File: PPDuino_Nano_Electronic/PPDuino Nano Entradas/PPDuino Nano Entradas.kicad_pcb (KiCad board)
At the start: 2 copper layers, 51.6 x 59.4 mm, 27 parts, among them J10 PWR_OUT, J11 INPUTS, J2 DI, J3 AI, U1 4N35, U2 4N35, U3 4N35, U4 4N35

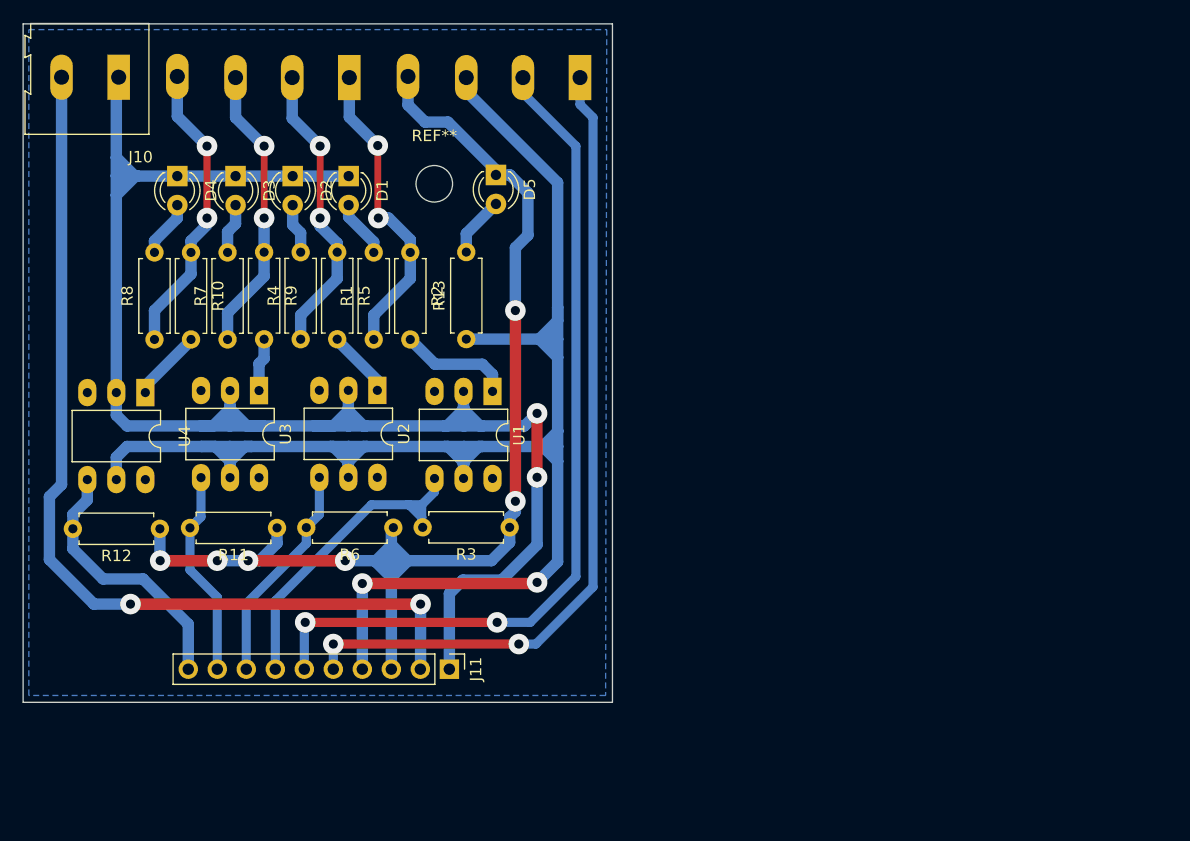
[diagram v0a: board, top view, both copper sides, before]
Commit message: Actualizar documentacion 2
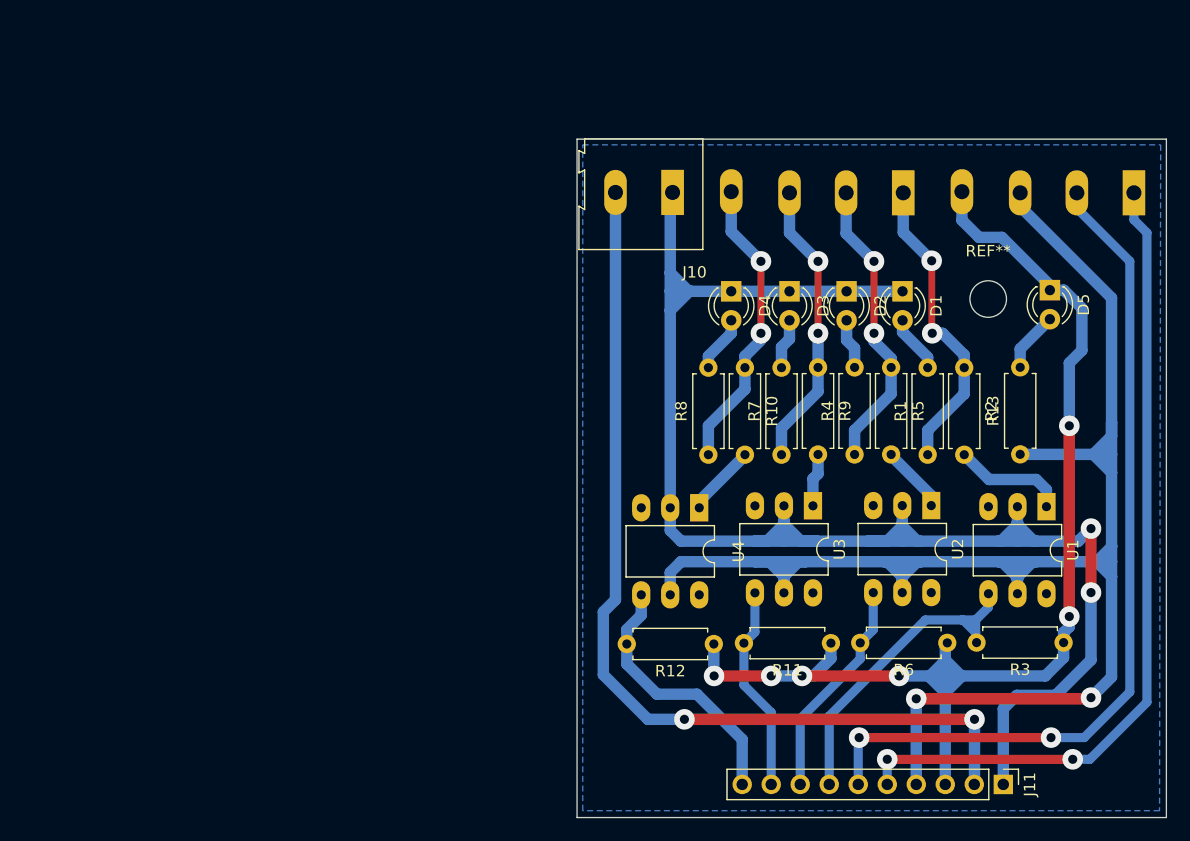
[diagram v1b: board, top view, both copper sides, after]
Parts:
- moved D5 49.5 mm to (161.3, 74.6)
- moved R2 49.5 mm to (153.8, 81.4)
- moved R7 49.5 mm to (137.8, 89.0)
- moved D1 49.5 mm to (148.4, 74.7)
- moved D2 49.5 mm to (143.5, 74.7)
- moved D3 49.5 mm to (138.5, 74.7)
- moved D4 49.5 mm to (133.4, 74.7)
- moved J11 49.5 mm to (157.2, 117.9)
- moved J2 49.5 mm to (148.5, 66.0)
- moved R1 49.5 mm to (150.6, 89.0)
- moved R10 49.5 mm to (134.6, 81.4)
- moved R11 49.5 mm to (142.1, 105.5)
- moved R12 49.5 mm to (131.9, 105.6)
- moved R3 49.5 mm to (162.5, 105.5)
- moved R5 49.5 mm to (147.4, 81.4)
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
